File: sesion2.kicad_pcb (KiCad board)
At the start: 2 copper layers, 45 x 35.5 mm, 14 parts, among them IC1 AT89LS51-16AU, J1 1366004, J2 68000-106HLF

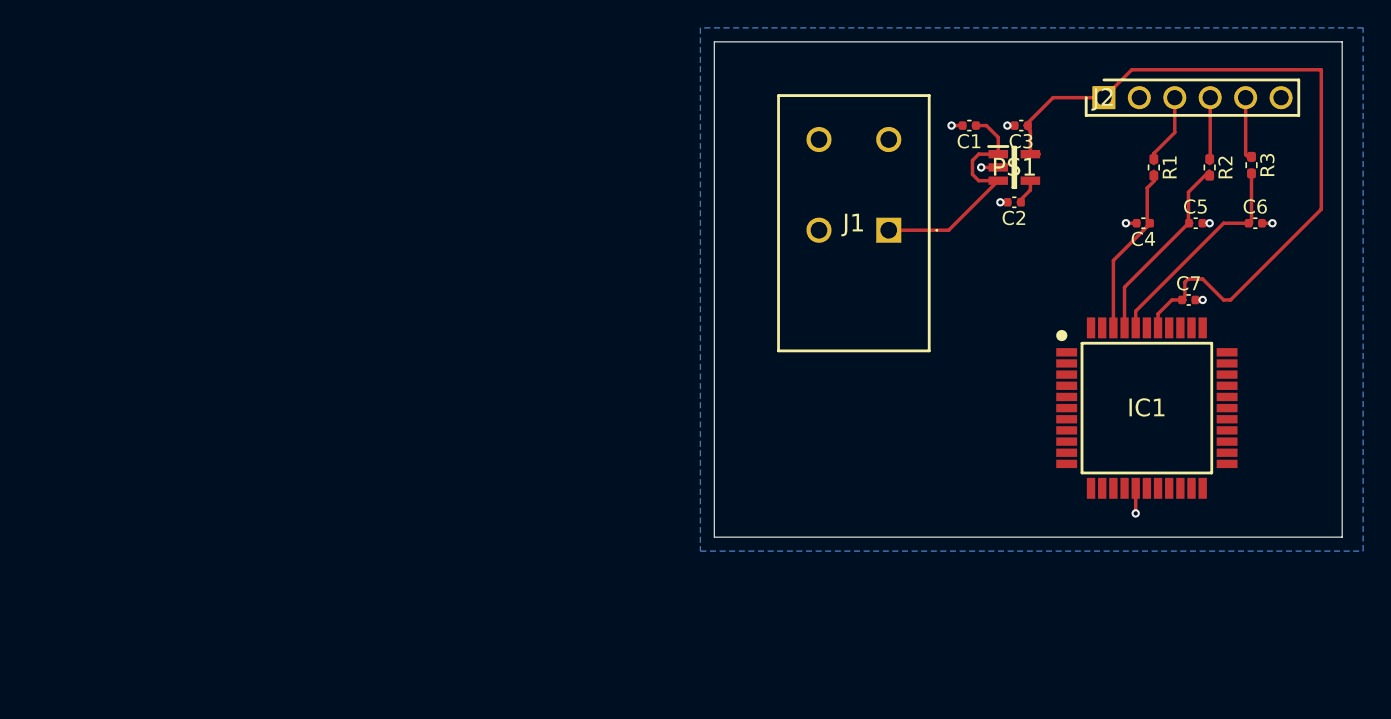
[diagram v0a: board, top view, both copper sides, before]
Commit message: Sesion4
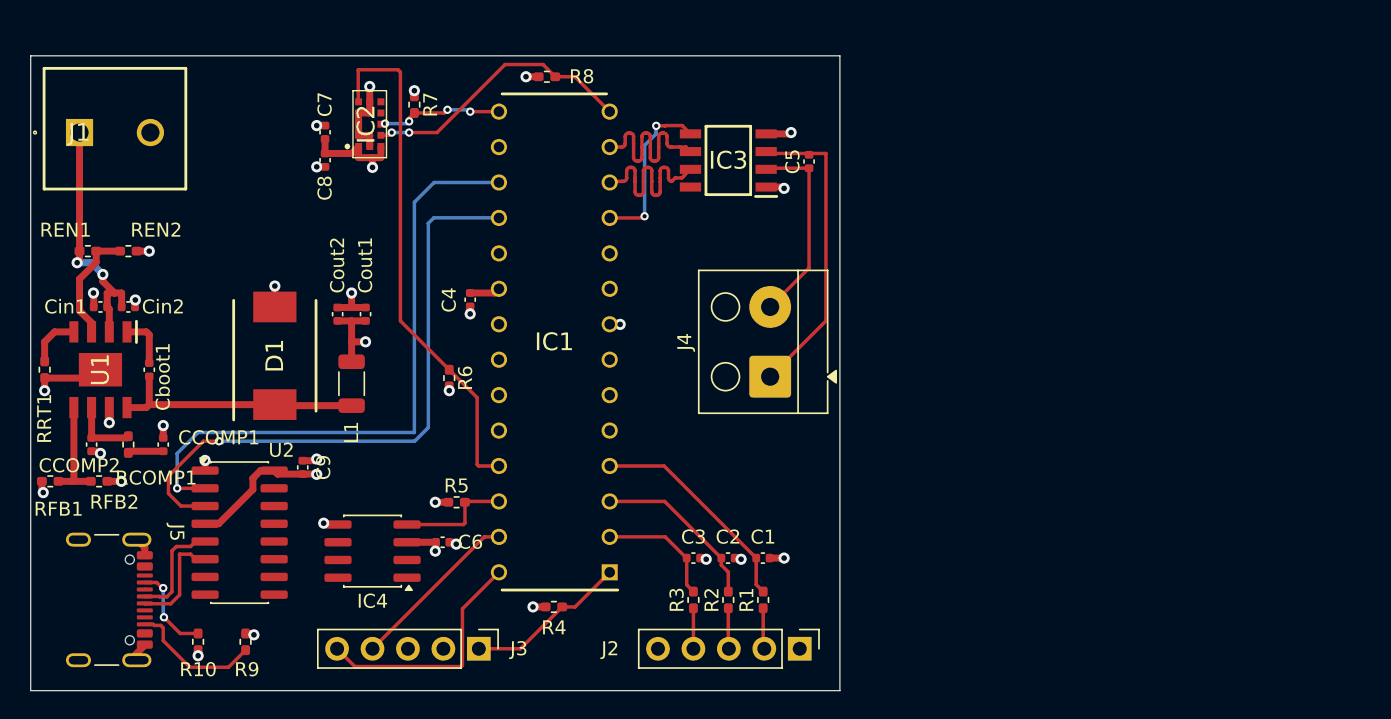
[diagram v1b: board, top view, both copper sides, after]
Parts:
- removed PS1: TAR5SB30_TE85L,F_, Samacsys:SOT95P275X140-5N
- added C8: 100 nF, Capacitor_SMD:C_0402_1005Metric, F.Cu at (94.1, 100.0)
- added C9: 100nF, Capacitor_SMD:C_0402_1005Metric, F.Cu at (92.5, 122.0)
- added CCOMP1: 82 nF, Capacitor_SMD:C_0402_1005Metric, F.Cu at (82.5, 120.4)
- added CCOMP2: 180pF, Capacitor_SMD:C_0402_1005Metric, F.Cu at (77.4, 120.4)
- added Cboot1: 100 nF, Capacitor_SMD:C_0402_1005Metric, F.Cu at (81.5, 115.0)
- added Cin1: 4.7 uF, Capacitor_SMD:C_0402_1005Metric, F.Cu at (78.0, 110.5)
- added Cin2: 4.7 uF, Capacitor_SMD:C_0402_1005Metric, F.Cu at (80.0, 110.5)
- added Cout1: 22 uF, Capacitor_SMD:C_0402_1005Metric, F.Cu at (97.0, 111.0)
- added Cout2: 22 uF, Capacitor_SMD:C_0402_1005Metric, F.Cu at (95.0, 111.0)
- added D1: B560C, Samacsys:DIOM7959X250N, F.Cu at (90.5, 114.0)
- added IC2: VL53L1CXV0FY_1, Samacsys:VL53L1CXV0FY1, F.Cu at (97.3, 97.4)
- added IC3: MAX31855SASA+T, Samacsys:SOIC127P600X175-8N, F.Cu at (123.0, 100.0)
- added IC4: DS18B20Z+, Package_SO:SOIC-8_3.9x4.9mm_P1.27mm, F.Cu at (97.5, 128.0)
- added J3: Conn_01x05, Connector_PinHeader_2.54mm:PinHeader_1x05_P2.54mm_Vertical, F.Cu at (105.1, 135.0)
- added J4: Conn_01x02, TerminalBlock_Altech:Altech_AK100_1x02_P5.00mm, F.Cu at (126.0, 115.5)
- added J5: USB_C_Receptacle_USB2.0_16P, Connector_USB:USB_C_Receptacle_GCT_USB4105-xx-A_16P_TopMnt_Horizontal, F.Cu at (77.5, 131.5)
- added L1: 10uH, Inductor_SMD:L_1206_3216Metric, F.Cu at (96.0, 116.0)
- added R10: 5.1k, Resistor_SMD:R_0402_1005Metric_Pad0.72x0.64mm_HandSolder, F.Cu at (85.0, 134.5)
- added R4: 10k, Resistor_SMD:R_0402_1005Metric_Pad0.72x0.64mm_HandSolder, F.Cu at (110.5, 132.0)
- added R5: 4.7k, Resistor_SMD:R_0402_1005Metric_Pad0.72x0.64mm_HandSolder, F.Cu at (103.5, 124.5)
- added R6: 3.3k, Resistor_SMD:R_0402_1005Metric_Pad0.72x0.64mm_HandSolder, F.Cu at (103.0, 115.6)
- added R7: 3.3k, Resistor_SMD:R_0402_1005Metric_Pad0.72x0.64mm_HandSolder, F.Cu at (100.5, 96.0)
- added R8: 3.3k, Resistor_SMD:R_0402_1005Metric_Pad0.72x0.64mm_HandSolder, F.Cu at (110.0, 94.0)
- added R9: 5.1k, Resistor_SMD:R_0402_1005Metric_Pad0.72x0.64mm_HandSolder, F.Cu at (88.4, 134.5)
- added RCOMP1: 3.24, Resistor_SMD:R_0402_1005Metric_Pad0.72x0.64mm_HandSolder, F.Cu at (80.0, 120.4)
- added REN1: 100k, Resistor_SMD:R_0402_1005Metric_Pad0.72x0.64mm_HandSolder, F.Cu at (77.1, 106.5)
- added REN2: 10k, Resistor_SMD:R_0402_1005Metric_Pad0.72x0.64mm_HandSolder, F.Cu at (80.0, 106.5)
- added RFB1: 31.2k, Resistor_SMD:R_0402_1005Metric_Pad0.72x0.64mm_HandSolder, F.Cu at (74.4, 123.0)
- added RFB2: 10k, Resistor_SMD:R_0402_1005Metric_Pad0.72x0.64mm_HandSolder, F.Cu at (77.9, 123.0)
- added RRT1: 340k, Resistor_SMD:R_0402_1005Metric_Pad0.72x0.64mm_HandSolder, F.Cu at (74.0, 115.0)
- added U1: TPS54360BDDA, Samacsys:SOIC127P600X170-9N, F.Cu at (78.0, 115.0)
- added U2: CH340C, Package_SO:SOIC-16_3.9x9.9mm_P1.27mm, F.Cu at (88.0, 126.7)
- C1: value 1uF -> 100nF
- C2: value 0.01uF -> 100nF
- C3: value 10uF -> 100nF
- C5: value 100nF -> 10 nF
- C6: value 100nF -> 100 nF
- C7: value 100nF -> 4.7 nF
- IC1: value AT89LS51-16AU -> PIC16F18855-I_SP; footprint Samacsys:QFP80P1200X1200X120-44N -> Samacsys:DIP794W56P254L3486H508Q28N
- J1: value 1366004 -> TB0012-508-02GR; footprint Samacsys:1366004 -> Samacsys:TB0012-508-02GR
- J2: value 68000-106HLF -> Conn_01x05; footprint Samacsys:HDRV6W64P0X254_1X6_1524X254X839P -> Connector_PinHeader_2.54mm:PinHeader_1x05_P2.54mm_Vertical
- R1, R2, R3: value 10k -> 1k
- moved C7 63.1 mm to (94.1, 98.0), turned to -90 degrees
- moved C6 62.6 mm to (102.5, 127.4)
- moved J1 58.4 mm to (76.5, 98.0)
- moved R3 50.7 mm to (120.5, 131.5), turned to 90 degrees
- moved C4 48.6 mm to (104.5, 110.0), turned to -90 degrees
- moved R2 46.4 mm to (123.0, 131.5), turned to 90 degrees
- moved J2 45.1 mm to (128.1, 135.0), turned to -90 degrees
- moved IC1 42.7 mm to (110.5, 113.0), turned to 180 degrees
- moved R1 41.8 mm to (125.5, 131.5), turned to 90 degrees
- moved C3 38.9 mm to (120.5, 128.5), turned to 0 degrees
- moved C1 34.3 mm to (125.5, 128.5), turned to 0 degrees
- moved C2 32.7 mm to (123.0, 128.5), turned to 0 degrees
- moved C5 28.1 mm to (128.8, 100.1), turned to 90 degrees
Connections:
- C1 pad 1: +9V -> Net-(IC1-RA2)
- C2 pad 1: Net-(PS1-NOISE) -> Net-(IC1-RA1)
- C3 pad 1: /Alimentacion/Vout3v -> Net-(IC1-RA0)
- C4 pad 1: Net-(IC1-P1.2) -> /Alimentacion/3.3v
- C5 pad 1: Net-(IC1-P1.1) -> Net-(IC3-T-)
- C5 pad 2: GND -> Net-(IC3-T+)
- C6 pad 1: Net-(IC1-P1.0) -> /Alimentacion/3.3v
- C7 pad 1: /Alimentacion/Vout3v -> GND
- C7 pad 2: GND -> /Alimentacion/3.3v
- IC1 pad 1: unconnected-(IC1-(MOSI)_P1.5-Pad1) -> /Microcontrolador/MCLR/VPP
- IC1 pad 11: unconnected-(IC1-(T1)_P3.5-Pad11) -> /Microcontrolador/SPI_SCK
- IC1 pad 12: unconnected-(IC1-(~{WR)_P3.6}-Pad12) -> /Microcontrolador/SPI_MISO
- IC1 pad 13: unconnected-(IC1-(~{RD)_P3.7}-Pad13) -> /Microcontrolador/SPI_CS
- IC1 pad 14: unconnected-(IC1-XTAL2-Pad14) -> /Microcontrolador/I2C_SCL
- IC1 pad 15: unconnected-(IC1-XTAL1-Pad15) -> /Microcontrolador/I2C_SDA
- IC1 pad 16: GND -> unconnected-(IC1-RC5-Pad16)
- IC1 pad 17: unconnected-(IC1-GND_2-Pad17) -> /Microcontrolador/UART_TX
- IC1 pad 18: unconnected-(IC1-(A8)_P2.0-Pad18) -> /Microcontrolador/UART_RX
- IC1 pad 19: unconnected-(IC1-(A9)_P2.1-Pad19) -> GND
- IC1 pad 2: unconnected-(IC1-(MISO)_P1.6-Pad2) -> Net-(IC1-RA0)
- IC1 pad 20: unconnected-(IC1-(A10)_P2.2-Pad20) -> /Alimentacion/3.3v
- IC1 pad 25: unconnected-(IC1-P2.7_(A15)-Pad25) -> /Microcontrolador/XHUT
- IC1 pad 26: unconnected-(IC1-~{PSEN}-Pad26) -> /Microcontrolador/DQ
- IC1 pad 27: unconnected-(IC1-ALE/~{PROG}-Pad27) -> /Microcontrolador/PGC
- IC1 pad 28: unconnected-(IC1-NC_2-Pad28) -> /Microcontrolador/PGD
- IC1 pad 3: unconnected-(IC1-(SCK)_P1.7-Pad3) -> Net-(IC1-RA1)
- IC1 pad 4: unconnected-(IC1-RST-Pad4) -> Net-(IC1-RA2)
- IC1 pad 8: unconnected-(IC1-(~{INT0)_P3.2}-Pad8) -> GND
- J1 pad 1: +9V -> Net-(U1-VIN)
- J2 pad 1: /Alimentacion/Vout3v -> GND
- J2 pad 2: GND -> Net-(J2-Pin_2)
- J2 pad 3: Net-(J2-Pad3) -> Net-(J2-Pin_3)
- J2 pad 4: Net-(J2-Pad4) -> Net-(J2-Pin_4)
- J2 pad 5: Net-(J2-Pad5) -> /Alimentacion/3.3v
- R1 pad 1: Net-(J2-Pad3) -> Net-(J2-Pin_2)
- R1 pad 2: Net-(IC1-P1.2) -> Net-(IC1-RA2)
- R2 pad 1: Net-(J2-Pad4) -> Net-(J2-Pin_3)
- R2 pad 2: Net-(IC1-P1.1) -> Net-(IC1-RA1)
- R3 pad 1: Net-(J2-Pad5) -> Net-(J2-Pin_4)
- R3 pad 2: Net-(IC1-P1.0) -> Net-(IC1-RA0)
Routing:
- net /Alimentacion/Vout3v: track 53.3 -> 0.00 mm
- net /Microcontrolador/UART_TX: track 0.00 -> 45.3 mm, vias 0 -> 1
- net /Microcontrolador/UART_RX: track 0.00 -> 44.2 mm, vias 0 -> 1
- net /Microcontrolador/XHUT: track 0.00 -> 37.4 mm
- net /Alimentacion/3.3v: track 0.00 -> 34.7 mm, vias 0 -> 11
- net GND: track 8.54 -> 34.7 mm, vias 9 -> 25
- net Net-(IC3-T+): track 0.00 -> 22.1 mm
- net /Microcontrolador/I2C_SCL: track 0.00 -> 19.9 mm, vias 0 -> 2
- net Net-(D1-K): track 0.00 -> 18.2 mm
- net Net-(U1-VIN): track 0.00 -> 18.1 mm, vias 0 -> 2
- net +9V: track 17.7 -> 0.00 mm
- net /Microcontrolador/PGD: track 0.00 -> 17.3 mm
- net Net-(IC1-P1.0): track 15.9 -> 0.00 mm
- net Net-(IC1-RA2): track 0.00 -> 15.8 mm
- net /Microcontrolador/SPI_MISO: track 0.00 -> 14.8 mm
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- added copper zone on In2.Cu, net /Alimentacion/3.3v
- added copper zone on In1.Cu, net GND
- removed copper zone on B.Cu, net GND
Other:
- board size 45 x 35.5 mm -> 58 x 45.5 mm
- copper layers 2 -> 4
